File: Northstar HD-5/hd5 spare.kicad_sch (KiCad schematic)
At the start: 9 parts, among them U1C1 74S10, U1F1 74S04, U1K1 LM393, U1L1 7438, U3D1 74LS04, U4D1 74S04, U4J1 74LS04, U5H1 74LS32, U5J1 74LS00

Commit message: placed components and repaired multi sheet labels
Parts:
- U1K1: footprint Package_DIP:DIP-8-16_W7.62mm -> Package_DIP:DIP-8_W7.62mm
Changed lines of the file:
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@@
     (property "Reference" "U1K1" (id 0) (at 166.37 88.1085 0))
     (property "Value" "LM393" (id 1) (at 166.37 90.8836 0))
-    (property "Footprint" "Package_DIP:DIP-8-16_W7.62mm" (id 2) (at 166.37 97.155 0)
+    (property "Footprint" "Package_DIP:DIP-8_W7.62mm" (id 2) (at 166.37 97.155 0)
       (effects (font (size 1.27 1.27)) hide)
     )

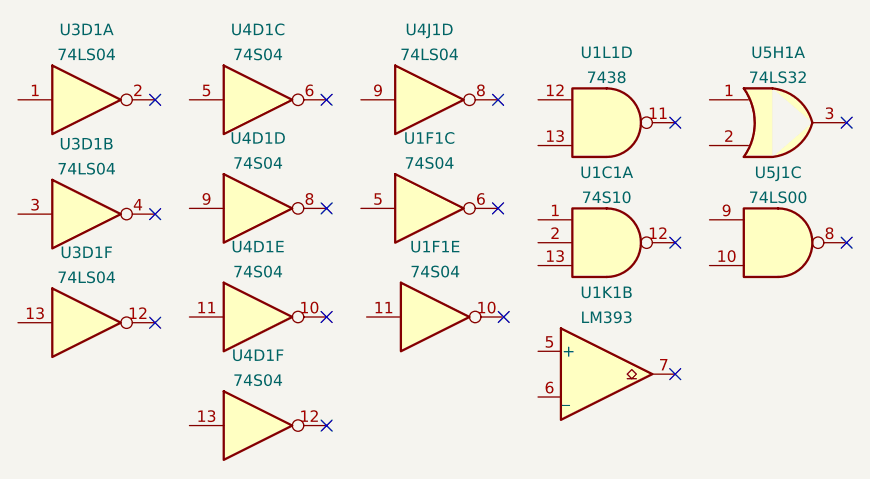
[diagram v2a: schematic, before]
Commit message: small updates to boards
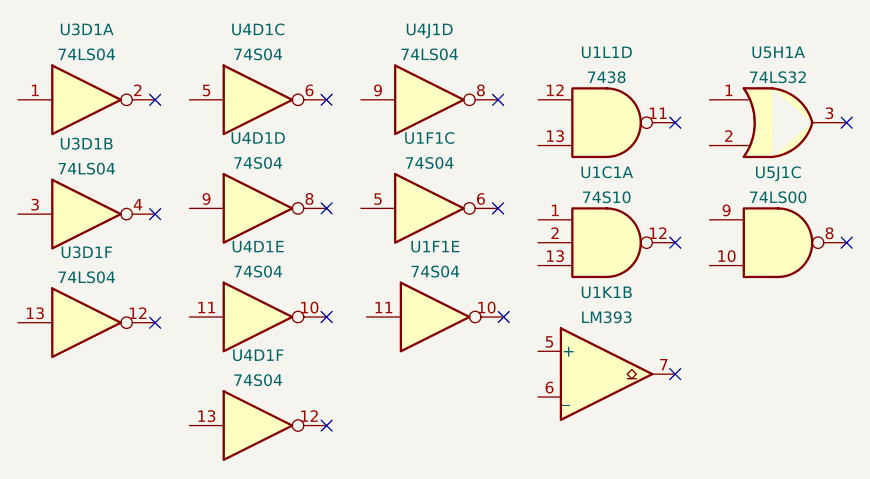
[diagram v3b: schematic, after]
